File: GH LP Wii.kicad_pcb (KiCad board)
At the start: 2 copper layers, 100 x 55 mm, 6 parts

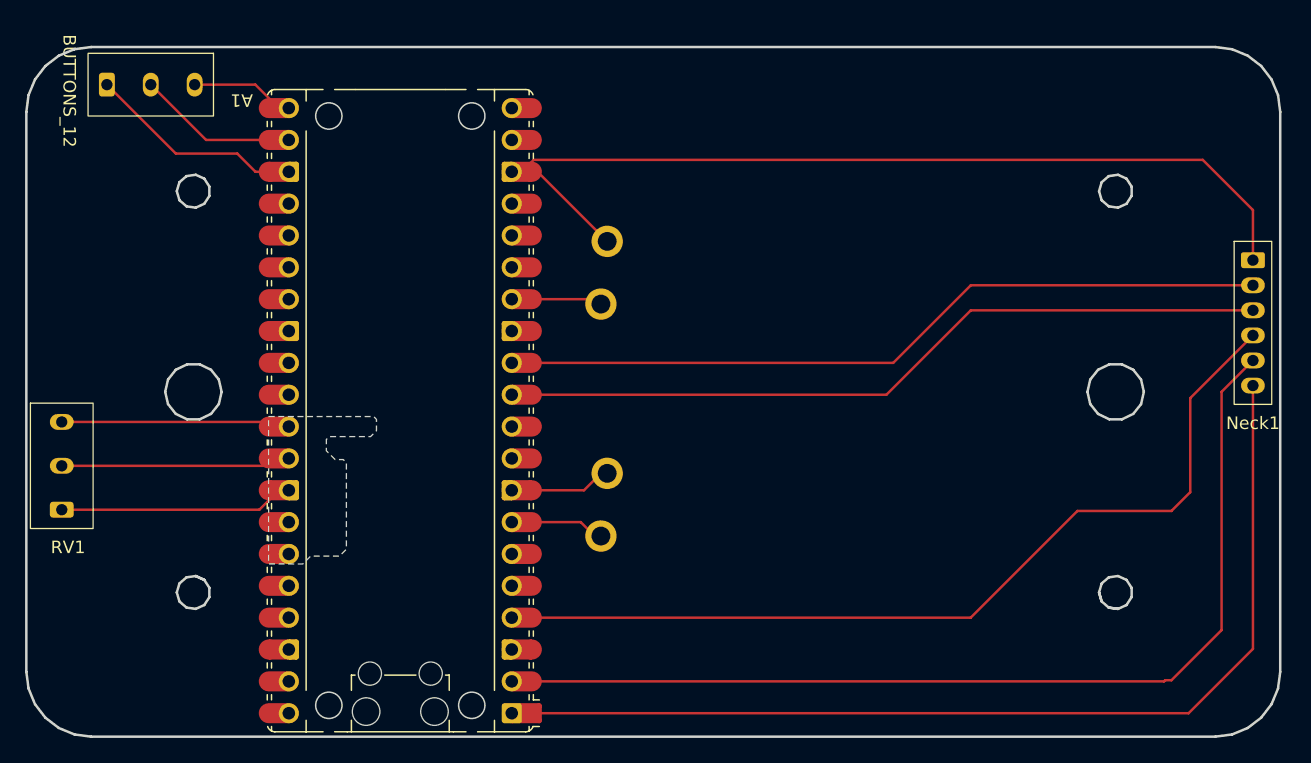
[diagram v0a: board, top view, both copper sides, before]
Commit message: gonna print
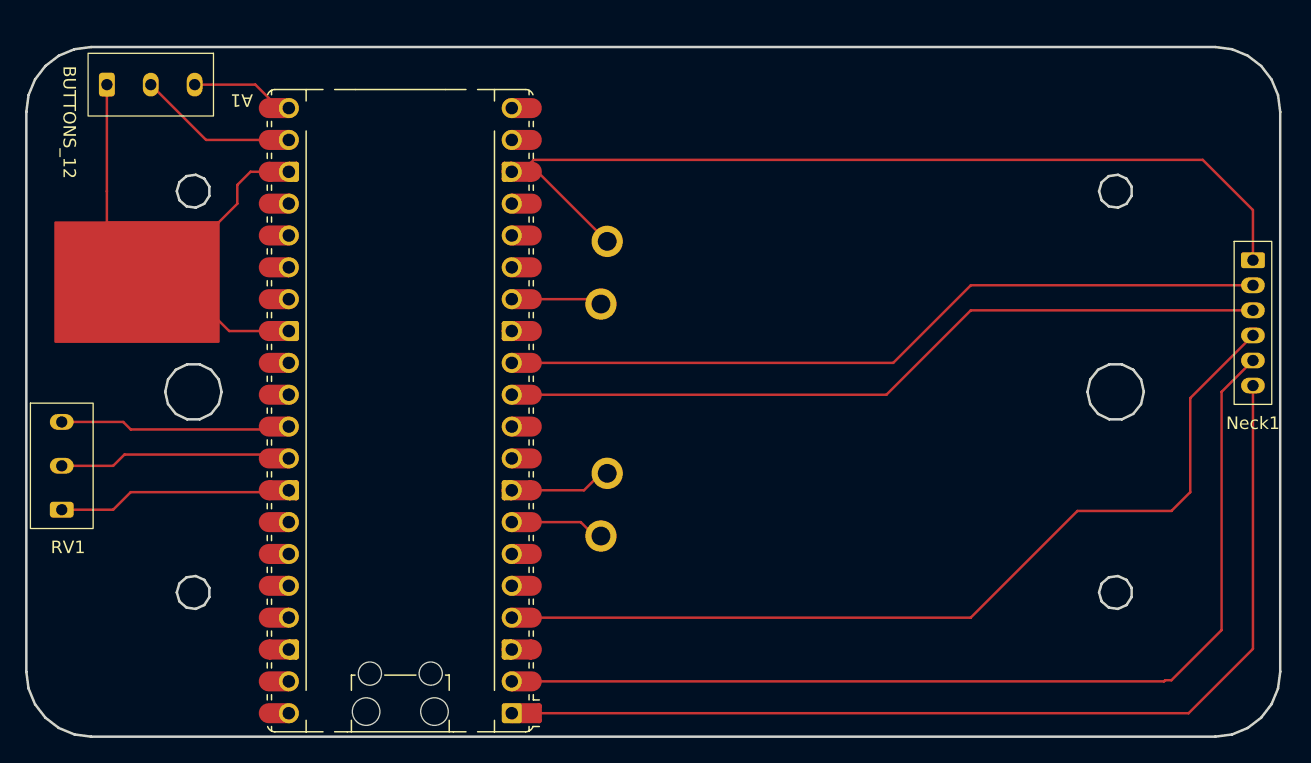
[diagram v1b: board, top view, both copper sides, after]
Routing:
- net Net-(Neck1-GND): track 97.4 -> 117.2 mm
- net Net-(A1-AGND): track 18.0 -> 16.6 mm
- net Net-(A1-GPIO26_ADC0): track 17.5 -> 16.7 mm

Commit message: Update settings and stuff
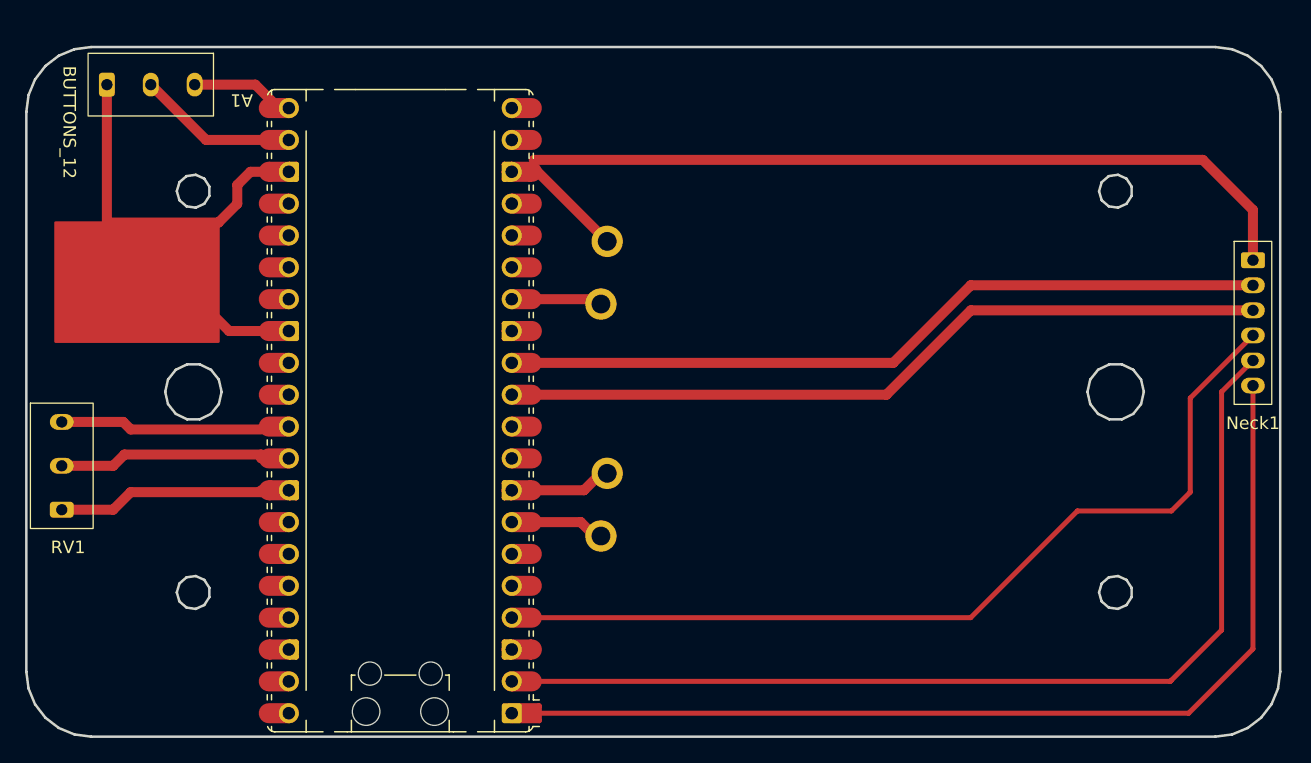
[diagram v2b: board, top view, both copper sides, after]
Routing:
- net Net-(Neck1-GND): track 117.2 -> 127.8 mm
